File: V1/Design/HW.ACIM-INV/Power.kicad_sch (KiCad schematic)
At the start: 42 parts, among them J1 HIGH VOLT, J4 LOW VOLT, U14 LDO 3.3V/1.5A, U18 LDO 3.3V/250mA, U8 LDO 3.3V±0.1%/20mA

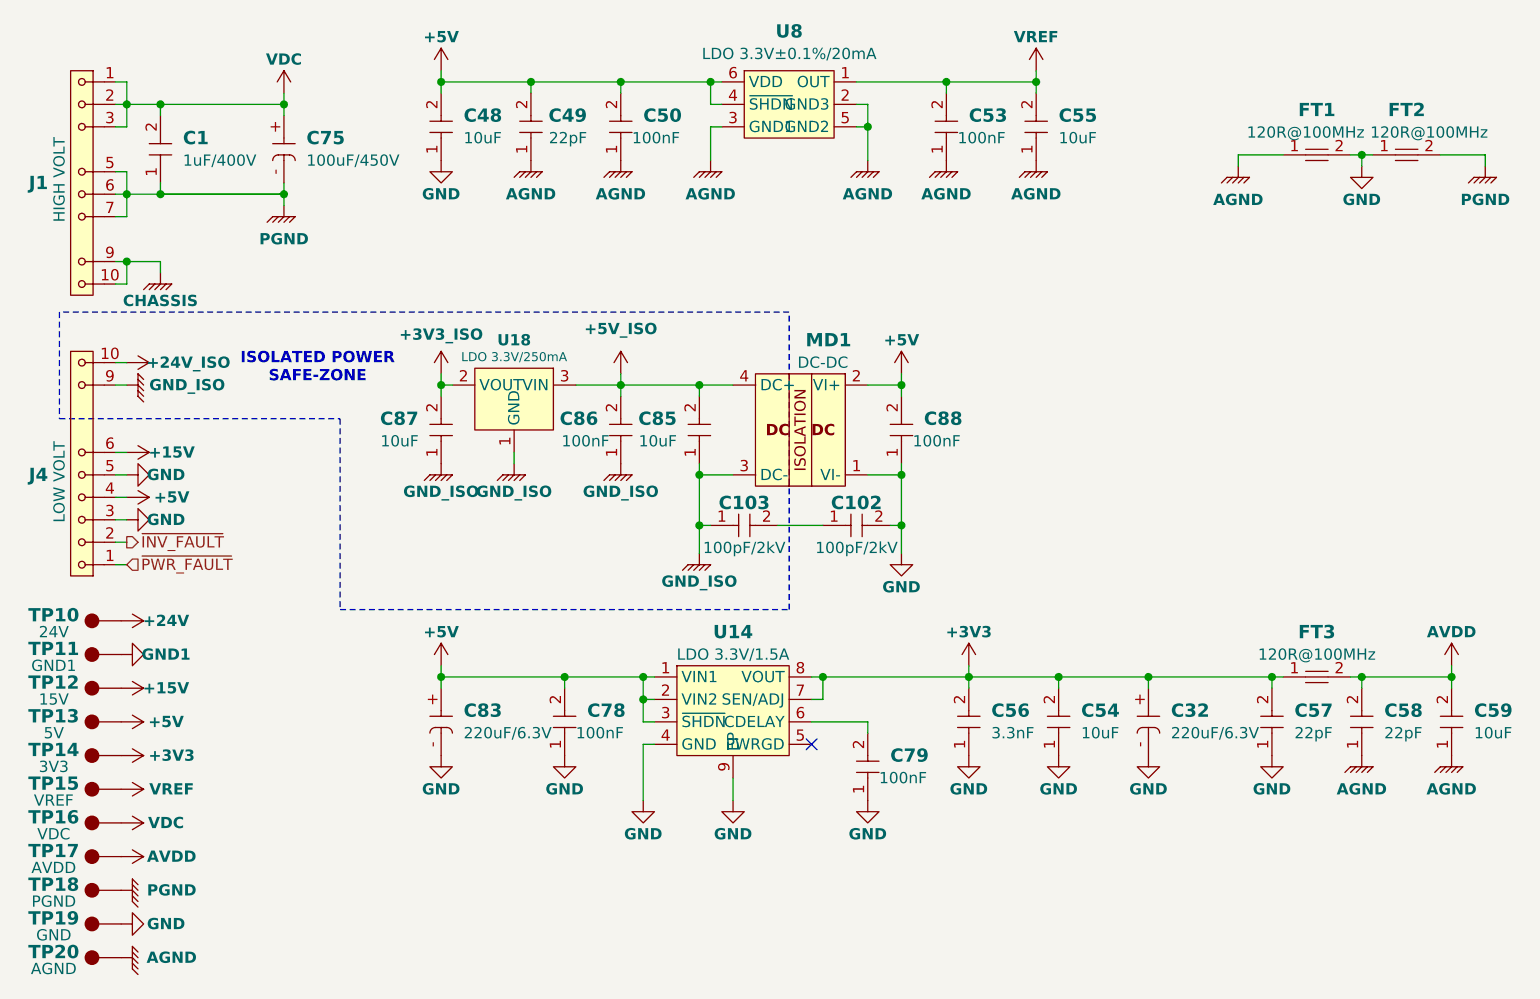
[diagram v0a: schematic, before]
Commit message: V1 schematic update 2
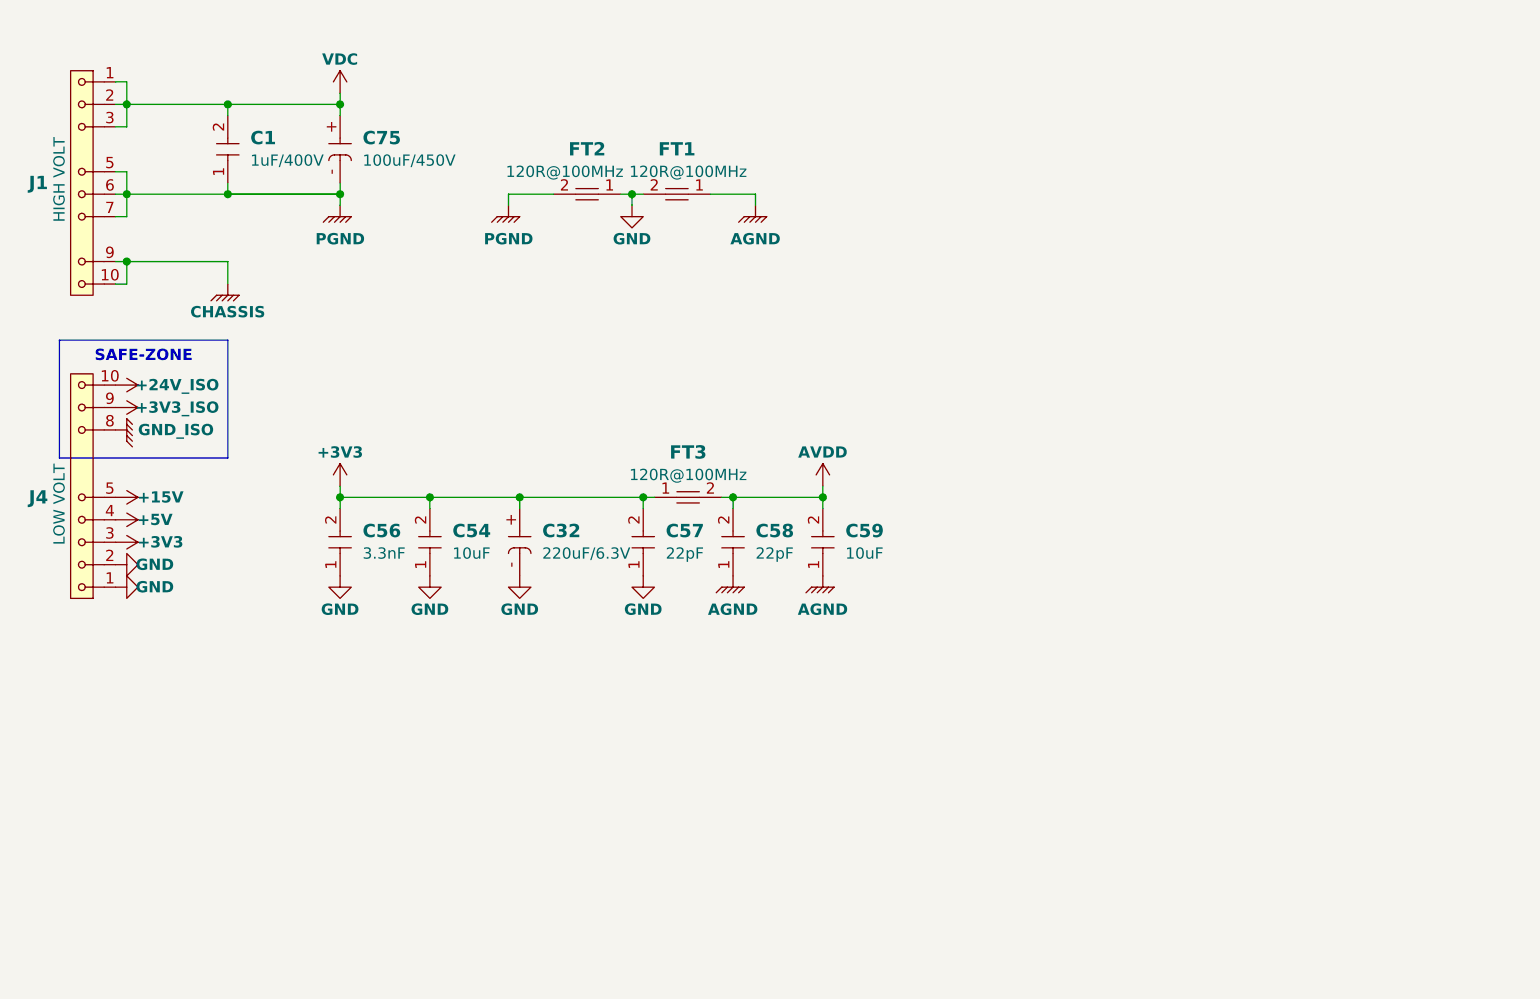
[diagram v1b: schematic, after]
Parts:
- removed C102, C103: 100pF/2kV, SAMPI:CAP1206, symbol SAMPI:CERCAP
- removed C48, C55, C85, C87: 10uF, SAMPI:CAP0603, symbol SAMPI:CERCAP
- removed C49: 22pF, SAMPI:CAP0603, symbol SAMPI:CERCAP
- removed C50, C53, C78, C79, C86, C88: 100nF, SAMPI:CAP0603, symbol SAMPI:CERCAP
- removed C83: 220uF/6.3V, SAMPI:CAP1411, symbol SAMPI:ELECCAP
- removed MD1: DC-DC, Liem:B1524S-1WR3, symbol SAMPI:DC-DC
- removed TP10: 24V, SAMPI:TP1MM, symbol SAMPI:TESTPOINT
- removed TP11: GND1, SAMPI:TP1MM, symbol SAMPI:TESTPOINT
- removed TP12: 15V, SAMPI:TP1MM, symbol SAMPI:TESTPOINT
- removed TP13: 5V, SAMPI:TP1MM, symbol SAMPI:TESTPOINT
- removed TP14: 3V3, SAMPI:TP1MM, symbol SAMPI:TESTPOINT
- removed TP15: VREF, SAMPI:TP1MM, symbol SAMPI:TESTPOINT
- removed TP16: VDC, SAMPI:TP1MM, symbol SAMPI:TESTPOINT
- removed TP17: AVDD, SAMPI:TP1MM, symbol SAMPI:TESTPOINT
- removed TP18: PGND, SAMPI:TP1MM, symbol SAMPI:TESTPOINT
- removed TP19: GND, SAMPI:TP1MM, symbol SAMPI:TESTPOINT
- removed TP20: AGND, SAMPI:TP1MM, symbol SAMPI:TESTPOINT
- removed U14: LDO 3.3V/1.5A, SAMPI:DFN8_3x3_MCHP, symbol SAMPI:MCP1727
- removed U18: LDO 3.3V/250mA, SAMPI:SOT23, symbol SAMPI:LDO
- removed U8: LDO 3.3V±0.1%/20mA, SAMPI:SOT-23-6_MCHP, symbol SAMPI:MCP1501
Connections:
- net ~{INV_FAULT} is gone; now on net GND: J4.2
- net ~{PWR_FAULT} is gone; now on net GND: J4.1
- net +15V: now also J4.5; no longer J4.6
- net +3V3: now also J4.3
- net +3V3_ISO: now also J4.9
- net GND: no longer J4.3, J4.5
- net GND_ISO: now also J4.8; no longer J4.9
- no-connect marks 1 -> 0
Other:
- note added: "SAFE-ZONE"
- note removed: "ISOLATED POWER SAFE-ZONE"
- moved on the sheet: C1, C32, C54, C56, C57, C58, C59, C75, FT1, FT2, FT3, J4

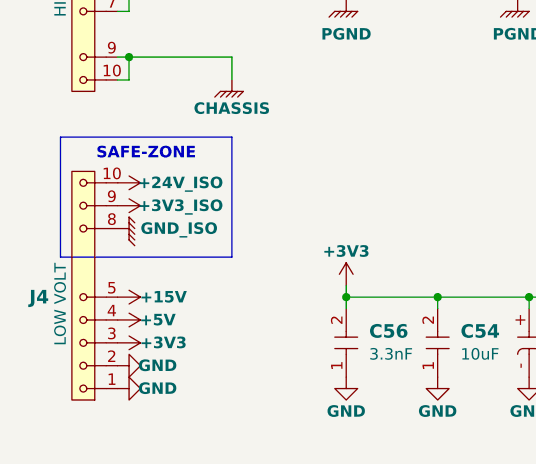
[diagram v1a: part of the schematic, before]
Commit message: V1 schematic update 3
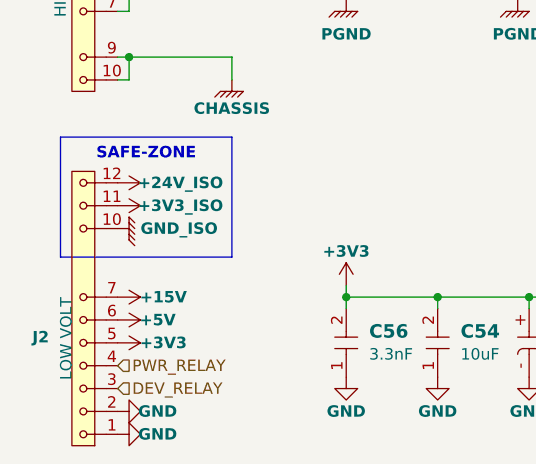
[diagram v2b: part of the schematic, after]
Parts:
- removed J4: LOW VOLT, SAMPI:HDM1x10x2.54_TH_RA, symbol SAMPI:SIL10
- added J2: LOW VOLT, symbol SAMPI:SIL12
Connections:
- net +15V: now also J2.7
- net +24V_ISO: now also J2.12
- net +3V3: now also J2.5
- net +3V3_ISO: now also J2.11
- net +5V: now also J2.6
- net GND: now also J2.1, J2.2
- net GND_ISO: now also J2.10
- new net DEV_RELAY: J2.3
- new net PWR_RELAY: J2.4
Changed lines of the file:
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@@
+		)
+	)
+	(hierarchical_label "DEV_RELAY"
+		(shape input)
+		(at 31.75 82.55 0)
+		(fields_autoplaced yes)
+		(effects
+			(font
+				(size 1.27 1.27)
+			)
+			(justify left)
+		)
+	)
+	(hierarchical_label "PWR_RELAY"
+		(shape input)
+		(at 31.75 80.01 0)
+		(fields_autoplaced yes)
+		(effects
+			(font
+				(size 1.27 1.27)
+			)
+			(justify left)
 		)
 	)
@@
 				(path "/20f80521-75f2-4ccc-bb34-c9566e70ef5c/34b63420-23a7-4d2d-affc-c07be2bf5f59"
 					(reference "#PWR0107")
-					(unit 1)
-				)
-			)
-		)
-	)
-	(symbol
-		(lib_id "SAMPI:SIL10")
-		(at 31.75 86.36 180)
-		(unit 1)
-		(exclude_from_sim no)
-		(in_bom yes)
-		(on_board yes)
-		(dnp no)
-		(property "Reference" "J4"
-			(at 24.13 72.39 0)
-			(effects
-				(font
-					(size 1.5 1.5)
-					(bold yes)
-				)
-				(justify left)
-			)
-		)
-		(property "Value" "LOW VOLT"
-			(at 25.4 68.58 90)
-			(effects
-				(font
-					(size 1.27 1.27)
-				)
-				(justify left)
-			)
-		)
-		(property "Footprint" "SAMPI:HDM1x10x2.54_TH_RA"
-			(at 31.75 86.36 0)
-			(effects
-				(font
-					(size 1.27 1.27)
-				)
-				(hide yes)
-			)
-		)
-		(property "Datasheet" ""
-			(at 31.75 86.36 0)
-			(effects
-				(font
-					(size 1.27 1.27)
-				)
-				(hide yes)
-			)
-		)
-		(property "Description" "CONN HDR 10POS 0.1 TIN PCB R/A"
-			(at 31.75 86.36 0)
-			(effects
-				(font
-					(size 1.27 1.27)
-				)
-				(hide yes)
-			)
-		)
-		(property "MFT" "Sullins"
-			(at 31.75 86.36 0)
-			(effects
-				(font
-					(size 1.27 1.27)
-				)
-				(hide yes)
-			)
-		)
-		(property "MNP" "PPTC101LGBN-RC"
-			(at 31.75 86.36 0)
-			(effects
-				(font
-					(size 1.27 1.27)
-				)
-				(hide yes)
-			)
-		)
-		(property "Checked" "OK"
-			(at 31.75 86.36 0)
-			(effects
-				(font
-					(size 1.27 1.27)
-				)
-				(hide yes)
-			)
-		)
-		(pin "8"
-		)
-		(pin "1"
-		)
-		(pin "2"
-		)
-		(pin "10"
-		)
-		(pin "4"
-		)
-		(pin "3"
-		)
-		(pin "9"
-		)
-		(pin "5"
-		)
-		(instances
-			(project "HW.ACIM-INV"
-				(path "/20f80521-75f2-4ccc-bb34-c9566e70ef5c/34b63420-23a7-4d2d-affc-c07be2bf5f59"
-					(reference "J4")
 					(unit 1)
 				)
@@
 	)
 	(symbol
+		(lib_id "SAMPI:SIL12")
+		(at 29.21 92.71 180)
+		(unit 1)
+		(exclude_from_sim no)
+		(in_bom yes)
+		(on_board yes)
+		(dnp no)
+		(property "Reference" "J2"
+			(at 24.13 76.835 0)
+			(effects
+				(font
+					(size 1.27 1.27)
+					(thickness 0.254)
+					(bold yes)
+				)
+				(justify left)
+			)
+		)
+		(property "Value" "LOW VOLT"
+			(at 26.035 72.3901 90)
+			(effects
+				(font
+					(size 1.27 1.27)
+				)
+				(justify left)
+			)
+		)
+		(property "Footprint" ""
+			(at 29.21 92.71 0)
+			(effects
+				(font
+					(size 1.27 1.27)
+				)
+				(hide yes)
+			)
+		)
+		(property "Datasheet" ""
+			(at 29.21 92.71 0)
+			(effects
+				(font
+					(size 1.27 1.27)
+				)
+				(hide yes)
+			)
+		)
+		(property "Description" ""
+			(at 29.21 92.71 0)
+			(effects
+				(font
+					(size 1.27 1.27)
+				)
+				(hide yes)
+			)
+		)
+		(pin "4"
+		)
+		(pin "3"
+		)
+		(pin "10"
+		)
+		(pin "2"
+		)
+		(pin "6"
+		)
+		(pin "1"
+		)
+		(pin "5"
+		)
+		(pin "7"
+		)
+		(pin "11"
+		)
+		(pin "12"
+		)
+		(instances
+			(project ""
+				(path "/20f80521-75f2-4ccc-bb34-c9566e70ef5c/34b63420-23a7-4d2d-affc-c07be2bf5f59"
+					(reference "J2")
+					(unit 1)
+				)
+			)
+		)
+	)
+	(symbol
 		(lib_id "power:GND")
 		(at 90.17 39.37 0)
@@
 	(symbol
 		(lib_id "power:GND")
-		(at 31.75 82.55 90)
+		(at 31.75 87.63 90)
 		(unit 1)
 		(exclude_from_sim no)
@@
 		(dnp no)
 		(property "Reference" "#PWR068"
-			(at 38.1 82.55 0)
+			(at 38.1 87.63 0)
 			(effects
 				(font
@@
 		)
 		(property "Value" "GND"
-			(at 36.195 82.55 90)
+			(at 36.195 87.63 90)
 			(effects
 				(font
@@
 		)
 		(property "Footprint" ""
-			(at 31.75 82.55 0)
-			(effects
-				(font
-					(size 1.27 1.27)
-				)
-				(hide yes)
-			)
-		)
-		(property "Datasheet" ""
-			(at 31.75 82.55 0)
+			(at 31.75 87.63 0)
+			(effects
+				(font
+					(size 1.27 1.27)
+				)
+				(hide yes)
+			)
+		)
+		(property "Datasheet" ""
+			(at 31.75 87.63 0)
 			(effects
 				(font
@@
 		)
 		(property "Description" ""
-			(at 31.75 82.55 0)
+			(at 31.75 87.63 0)
 			(effects
 				(font
@@
 	(symbol
 		(lib_id "power:GND")
-		(at 31.75 80.01 90)
+		(at 31.75 85.09 90)
 		(unit 1)
 		(exclude_from_sim no)
@@
 		(dnp no)
 		(property "Reference" "#PWR064"
-			(at 38.1 80.01 0)
+			(at 38.1 85.09 0)
 			(effects
 				(font
@@
 		)
 		(property "Value" "GND"
-			(at 36.195 80.01 90)
+			(at 36.195 85.09 90)
 			(effects
 				(font
@@
 		)
 		(property "Footprint" ""
-			(at 31.75 80.01 0)
-			(effects
-				(font
-					(size 1.27 1.27)
-				)
-				(hide yes)
-			)
-		)
-		(property "Datasheet" ""
-			(at 31.75 80.01 0)
+			(at 31.75 85.09 0)
+			(effects
+				(font
+					(size 1.27 1.27)
+				)
+				(hide yes)
+			)
+		)
+		(property "Datasheet" ""
+			(at 31.75 85.09 0)
 			(effects
 				(font
@@
 		)
 		(property "Description" ""
-			(at 31.75 80.01 0)
-			(effects
-				(font
+			(at 31.75 85.09 0)
+			(effects
+				(font
